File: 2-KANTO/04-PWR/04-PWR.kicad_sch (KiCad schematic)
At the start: 34 parts, among them J1 MAIN Conn, J2 voltmeter, J3 Battery, J4 OpenMV Conn, J5 Conn_01x20, J6 Conn_01x20, M1 ServoBasketLeft, M2 ServoBasketRight, M3 ServoArmLeft, M4 ServoArmRight, M5 ServoHandLeft, M6 ServoHandRight, Q1 Q_PMOS_GDS, SW1 SW_SPDT, SW2 SW_SPST, U3 RASPBERRY_PI_PICO

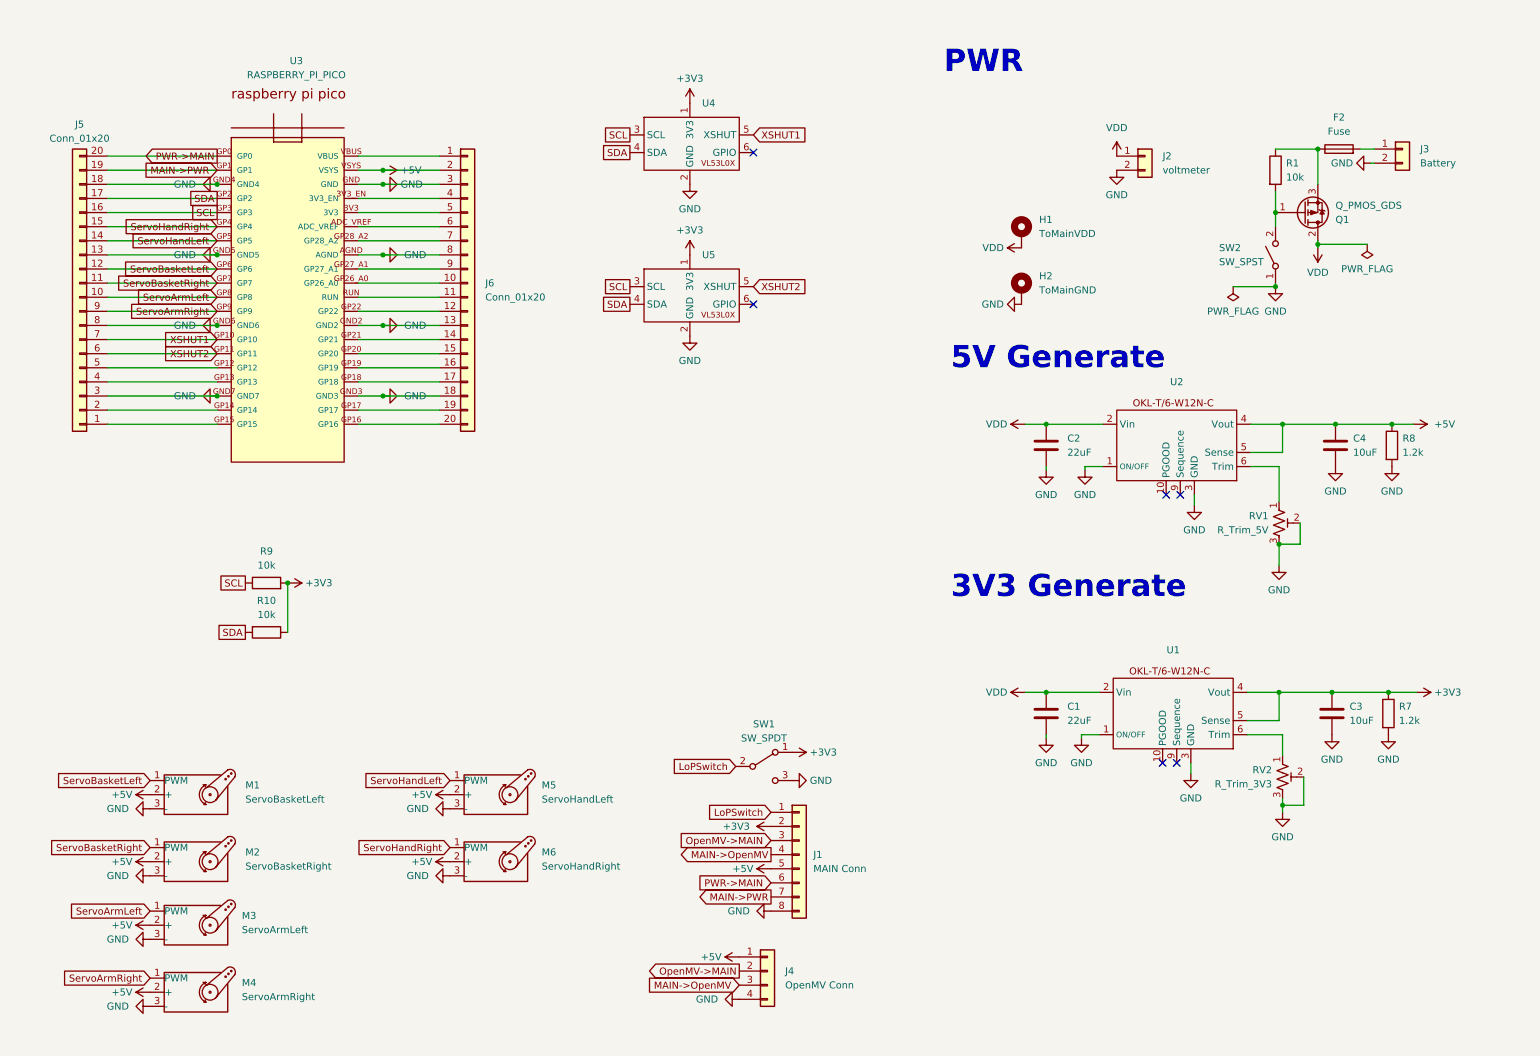
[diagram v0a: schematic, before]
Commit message: mike
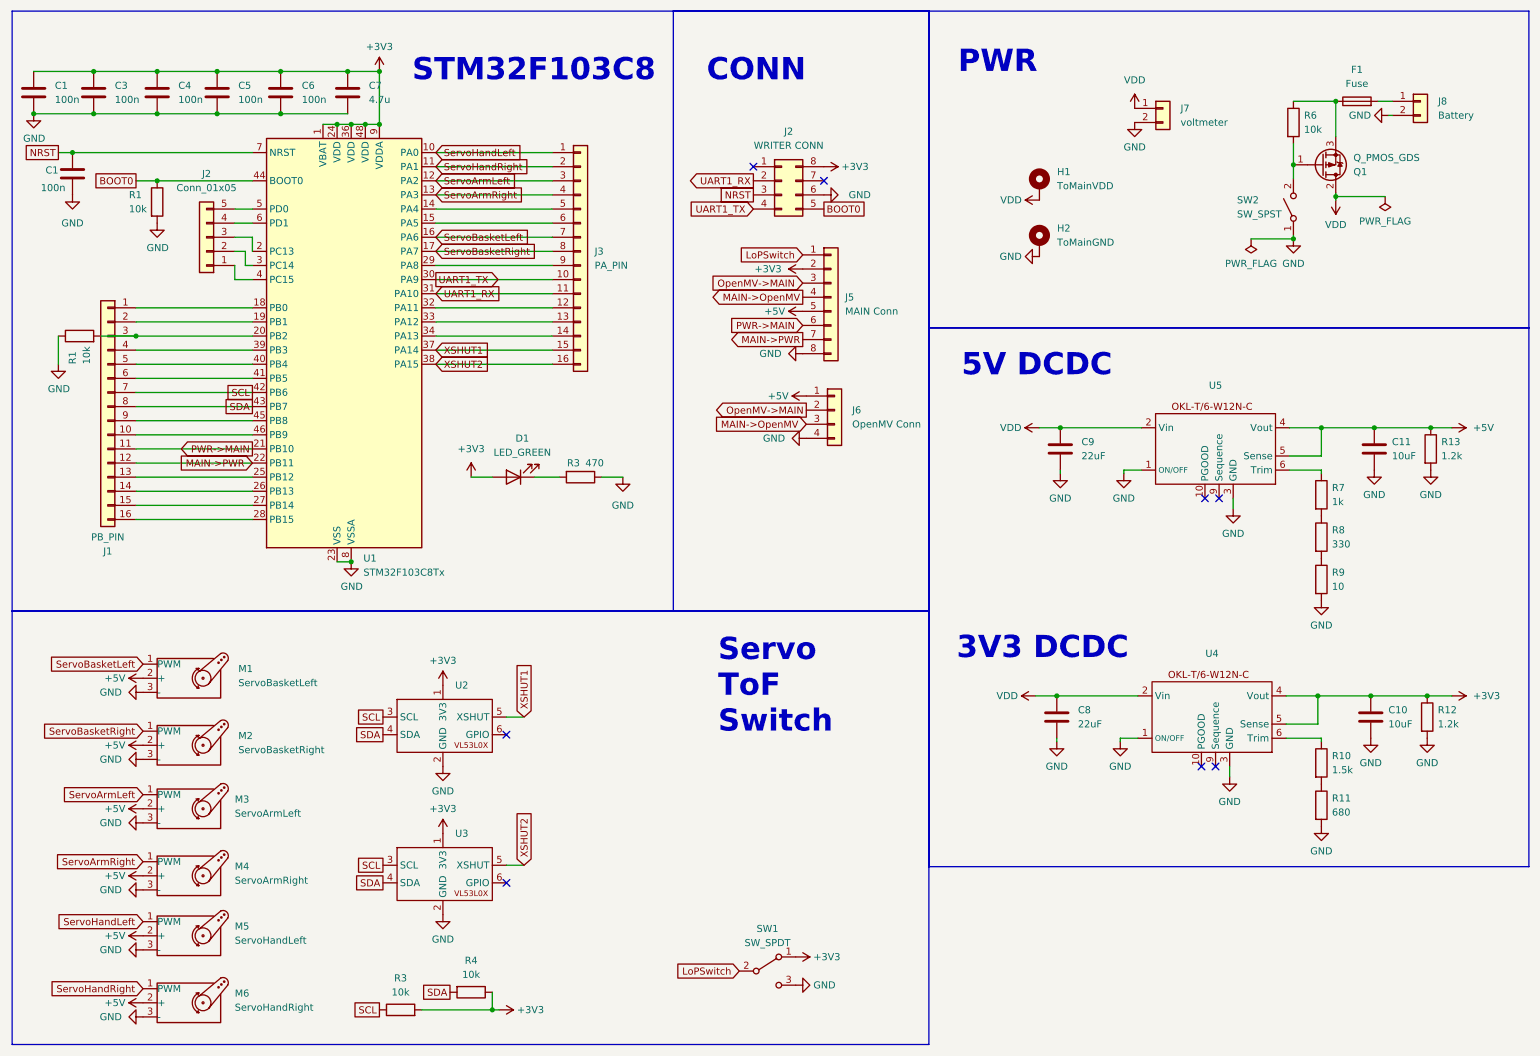
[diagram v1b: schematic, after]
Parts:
- removed C1, C2: 22uF, Capacitor_SMD:C_0805_2012Metric_Pad1.18x1.45mm_HandSolder, symbol Device:C
- removed J5, J6: Conn_01x20, Connector_PinHeader_2.54mm:PinHeader_1x20_P2.54mm_Vertical, symbol Connector_Generic:Conn_01x20
- removed RV1: R_Trim_5V, Potentiometer_THT:Potentiometer_Bourns_3006P_Horizontal, symbol Device:R_Potentiometer_Trim_US
- removed RV2: R_Trim_3V3, Potentiometer_THT:Potentiometer_Bourns_3006P_Horizontal, symbol Device:R_Potentiometer_Trim_US
- removed U1, U2: ~, Akiduki:OKL-T6-W12N-C-SMD, symbol akiduki:OKL-T/6-W12N-C
- removed U3: RASPBERRY_PI_PICO, Akiduki:RASPBERRY_PI_PICO, symbol akiduki:RASPBERRY_PI_PICO
- added C1 (x2), C5, C6: 100n, Capacitor_SMD:C_0402_1005Metric, symbol Device:C
- added C10, C11: 10uF, Capacitor_SMD:C_0805_2012Metric, symbol Device:C
- added C7: 4.7u, Resistor_SMD:R_0402_1005Metric, symbol Device:C
- added C8, C9: 22uF, Capacitor_SMD:C_0805_2012Metric, symbol Device:C
- added D1: LED_GREEN, LED_SMD:LED_0805_2012Metric, symbol Device:LED
- added J1: PB_PIN, Connector_PinHeader_2.54mm:PinHeader_1x16_P2.54mm_Vertical, symbol Connector_Generic:Conn_01x16
- added J2: Conn_01x05, Connector_PinHeader_2.54mm:PinHeader_1x05_P2.54mm_Vertical, symbol Connector_Generic:Conn_01x05
- added J2: WRITER CONN, Connector_PinSocket_2.54mm:PinSocket_2x04_P2.54mm_Horizontal, symbol Connector_Generic:Conn_02x04_Counter_Clockwise
- added J3: PA_PIN, Connector_PinHeader_2.54mm:PinHeader_1x16_P2.54mm_Vertical, symbol Connector_Generic:Conn_01x16
- added R1 (x2): 10k, Resistor_SMD:R_0603_1608Metric, symbol Device:R
- added R10: 1.5k, Resistor_SMD:R_0603_1608Metric, symbol Device:R
- added R11: 680, Resistor_SMD:R_0603_1608Metric, symbol Device:R
- added R12, R13: 1.2k, Resistor_SMD:R_0603_1608Metric, symbol Device:R
- added R3: 470, Resistor_SMD:R_0603_1608Metric, symbol Device:R
- added R9: 10, Resistor_SMD:R_0603_1608Metric, symbol Device:R
- added U1: STM32F103C8Tx, Package_QFP:LQFP-48_7x7mm_P0.5mm, symbol MCU_ST_STM32F1:STM32F103C8Tx
- added U4, U5: ~, Akiduki:OKL-T6-W12N-C-SMD, symbol akiduki:OKL-T/6-W12N-C
- C3, C4: value 10uF -> 100n; footprint Capacitor_SMD:C_1206_3216Metric_Pad1.33x1.80mm_HandSolder -> Capacitor_SMD:C_0402_1005Metric; LCSC C15850 -> C1525
- J5: renamed from J1; footprint Connector_JST:JST_XH_B8B-XH-A_1x08_P2.50mm_Vertical -> Connector_JST:JST_XH_S8B-XH-A_1x08_P2.50mm_Horizontal
- J6: renamed from J4; footprint Connector_JST:JST_XH_B4B-XH-A_1x04_P2.50mm_Vertical -> Connector_JST:JST_XH_S4B-XH-A_1x04_P2.50mm_Horizontal
- J7: renamed from J2; footprint Connector_Wire:SolderWire-0.5sqmm_1x02_P4.6mm_D0.9mm_OD2.1mm -> Connector_JST:JST_XH_S2B-XH-A_1x02_P2.50mm_Horizontal
- M1, M2: footprint Connector_PinHeader_2.54mm:PinHeader_1x03_P2.54mm_Horizontal -> Connector_PinHeader_2.54mm:PinHeader_1x03_P2.54mm_Vertical
- R3: renamed from R9; footprint Resistor_THT:R_Axial_DIN0207_L6.3mm_D2.5mm_P10.16mm_Horizontal -> Resistor_SMD:R_0603_1608Metric; LCSC (none) -> C25804
- R4: renamed from R10; footprint Resistor_THT:R_Axial_DIN0207_L6.3mm_D2.5mm_P10.16mm_Horizontal -> Resistor_SMD:R_0603_1608Metric; LCSC (none) -> C25804
- R6: renamed from R1; footprint Resistor_THT:R_Axial_DIN0207_L6.3mm_D2.5mm_P10.16mm_Horizontal -> Resistor_SMD:R_0603_1608Metric
- R7: value 1.2k -> 1k; footprint Resistor_THT:R_Axial_DIN0207_L6.3mm_D2.5mm_P10.16mm_Horizontal -> Resistor_SMD:R_0603_1608Metric; LCSC C22765 -> C21190
- R8: value 1.2k -> 330; footprint Resistor_THT:R_Axial_DIN0207_L6.3mm_D2.5mm_P10.16mm_Horizontal -> Resistor_SMD:R_0603_1608Metric; LCSC C22765 -> C23138
- SW1: footprint Connector_PinHeader_2.54mm:PinHeader_1x03_P2.54mm_Vertical -> Akiduki:SK-12D11VG3
- renumbered F2 to F1, J3 to J8, U4 to U2, U5 to U3
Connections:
- net +3V3: now also C4.1, C1.1, C10.1, C5.1, C6.1, C7.1, D1.2 (A), J2.8 (Pin_8), R12.1, U1.1 (VBAT), U1.24 (VDD), U1.36 (VDD), U1.48 (VDD), U1.9 (VDDA), U4.4 (Vout), U4.5 (Sense); no longer R7.1
- net +5V: now also C11.1, R13.1, U5.4 (Vout), U5.5 (Sense); no longer C4.1, R8.1
- net GND: now also C1.1, C1.2, C10.2, C11.2, C5.2, C6.2, C7.2, C8.2, C9.2, J2.6 (Pin_6), R1.1, R1.2, R11.2, R12.2, R13.2, R3.1, R9.2, U1.23 (VSS), U1.35 (VSS), U1.47 (VSS), U1.8 (VSSA), U4.1 (ON/OFF), U4.3 (GND), U4.7 (GND), U5.1 (ON/OFF), U5.3 (GND), U5.7 (GND); no longer R7.2, R8.2
- net MAIN->PWR: now also J1.12 (Pin_12), U1.22 (PB11)
- net PWR->MAIN: now also J1.11 (Pin_11), U1.21 (PB10)
- net SCL: now also J1.7 (Pin_7), U1.42 (PB6)
- net SDA: now also J1.8 (Pin_8), U1.43 (PB7)
- net ServoArmLeft: now also J3.3 (Pin_3), U1.12 (PA2)
- net ServoArmRight: now also J3.4 (Pin_4), U1.13 (PA3)
- net ServoBasketLeft: now also J3.7 (Pin_7), U1.16 (PA6)
- net ServoBasketRight: now also J3.8 (Pin_8), U1.17 (PA7)
- net ServoHandLeft: now also J3.1 (Pin_1), U1.10 (PA0)
- net ServoHandRight: now also J3.2 (Pin_2), U1.11 (PA1)
- net VDD: now also C8.1, C9.1, U4.2 (Vin), U5.2 (Vin)
- net XSHUT1: now also J3.15 (Pin_15), U1.37 (PA14)
- net XSHUT2: now also J3.16 (Pin_16), U1.38 (PA15)
- new net: J3.12 (Pin_12), U1.32 (PA11)
- new net: J3.13 (Pin_13), U1.33 (PA12)
- new net: J3.14 (Pin_14), U1.34 (PA13)
- new net: J3.5 (Pin_5), U1.14 (PA4)
- new net: J3.6 (Pin_6), U1.15 (PA5)
- new net: J3.9 (Pin_9), U1.29 (PA8)
- new net: J1.1 (Pin_1), U1.18 (PB0)
- new net: J1.10 (Pin_10), U1.46 (PB9)
- new net: J1.13 (Pin_13), U1.25 (PB12)
- new net: J1.14 (Pin_14), U1.26 (PB13)
- new net: J1.15 (Pin_15), U1.27 (PB14)
- new net: J1.16 (Pin_16), U1.28 (PB15)
- new net: J1.2 (Pin_2), U1.19 (PB1)
- new net: J1.3 (Pin_3), R1.2, U1.20 (PB2)
- new net: J1.4 (Pin_4), U1.39 (PB3)
- new net: J1.5 (Pin_5), U1.40 (PB4)
- new net: J1.6 (Pin_6), U1.41 (PB5)
- new net: J1.9 (Pin_9), U1.45 (PB8)
- new net: J2.1 (Pin_1), U1.4 (PC15)
- new net: J2.2 (Pin_2), U1.3 (PC14)
- new net: J2.3 (Pin_3), U1.2 (PC13)
- new net: J2.4 (Pin_4), U1.6 (PD1)
- new net: J2.5 (Pin_5), U1.5 (PD0)
- new net: R7.1, U5.6 (Trim)
- new net: R7.2, R8.1
- new net: R8.2, R9.1
- new net: D1.1 (K), R3.2
- new net: R10.1, U4.6 (Trim)
- new net: R10.2, R11.1
- new net BOOT0: J2.5 (Pin_5), R1.1, U1.44 (BOOT0)
- new net NRST: C1.2, J2.3 (Pin_3), U1.7 (NRST)
- new net UART1_RX: J2.2 (Pin_2), J3.11 (Pin_11), U1.31 (PA10)
- new net UART1_TX: J2.4 (Pin_4), J3.10 (Pin_10), U1.30 (PA9)
- no-connect marks 6 -> 8
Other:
- note added: "3V3 DCDC"
- note added: "5V DCDC"
- note added: "CONN"
- note added: "STM32F103C8"
- note added: "Servo ToF Switch"
- note removed: "3V3 Generate"
- note removed: "5V Generate"
- company: (none) -> Tuton
- title: (none) -> 04-PWR
- moved on the sheet: F1, H1, H2, J5, J6, J7, J8, M1, M2, M3, M4, M5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
